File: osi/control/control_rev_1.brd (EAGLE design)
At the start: 25.4 x 25.4 mm, 8 parts, among them IC1 TINY24/44/84-PU

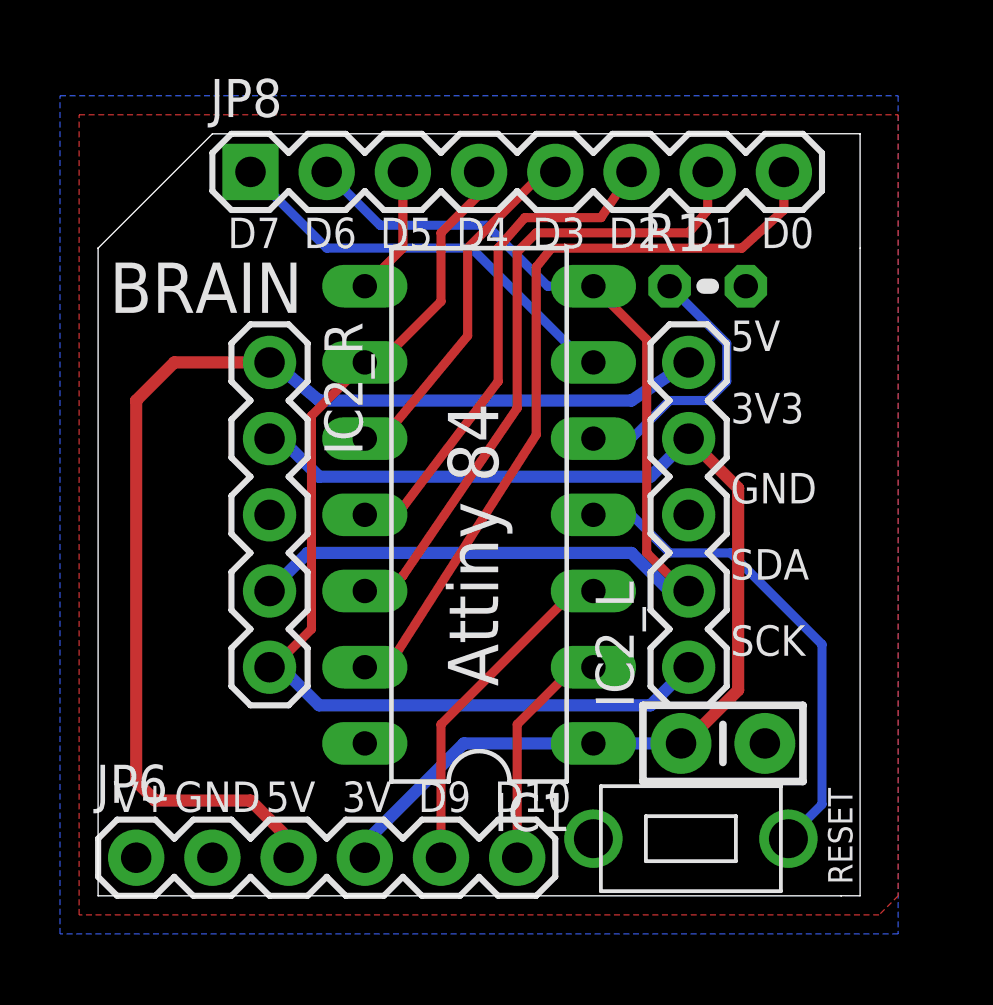
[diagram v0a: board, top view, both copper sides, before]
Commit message: control brain
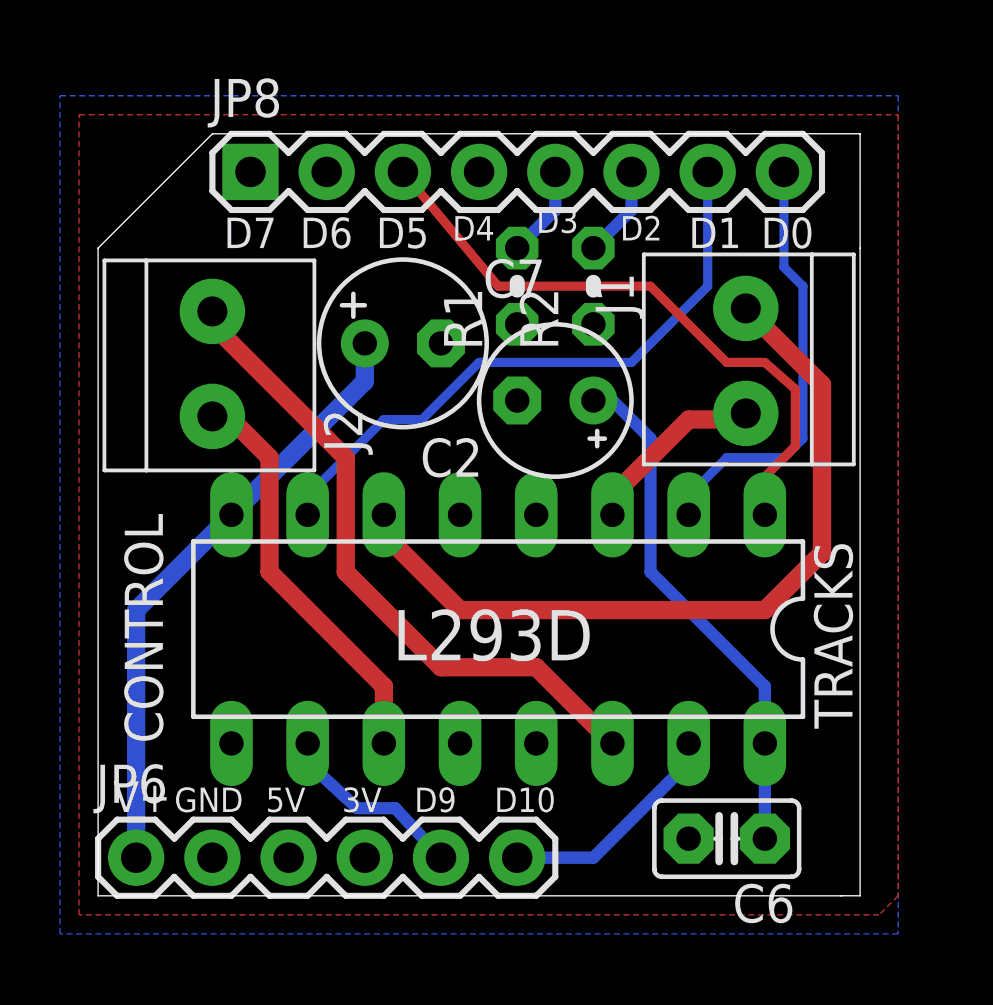
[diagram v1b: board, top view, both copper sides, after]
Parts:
- removed C1: (no value), SparkFun:CAP-PTH-SMALL-KIT
- removed IC1: TINY24/44/84-PU, avr-7:DIL14
- removed IC2_L, IC2_R: (no value), SparkFun_mod:1X05
- removed U$1: PTS635_SWITCH, _my-parts:PTS635_SWITCH
- added C2: 100uF/6V, rcl-ez:E2,5-5
- added C6: 0.1uF, rcl-ez:C025-025X050
- added C7: 100uF/16V, rcl-ez:E2,5-6
- added J1, J2: 1X2-3.5MM, adafruit_mod:1X2-3.5MM
- added R2: (no value), adafruit_mod:0204V
- added TRACKS: L293D, texas:DIL16
- moved R1 6.35 mm to (14.0, 20.3), turned to 90 degrees
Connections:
- removed net D8: IC1.5, R1.1
- removed net RESET: IC1.4, U$1.P$2
- new net N$1: J1.2, TRACKS.3
- new net N$2: J2.2, TRACKS.14
- new net N$3: J1.1, TRACKS.6
- new net N$4: J2.1, TRACKS.11
- new net N$5: TRACKS.9
- new net N$6: R1.1
- new net N$7: R2.1
- new net VCC: C2.+, C6.1, TRACKS.16
- net +3V3: no longer C1.2, IC1.1, IC2_L.4, IC2_R.2
- net +5V: no longer IC2_L.5, IC2_R.1
- net AREF_D0: now also TRACKS.2; no longer IC1.13
- net D1: now also TRACKS.7; no longer IC1.12
- net D10: now also TRACKS.15; no longer IC1.2
- net D2: now also R2.2; no longer IC1.11
- net D3: now also R1.2; no longer IC1.10
- net D5: now also TRACKS.1; no longer IC1.8
- net D7: no longer IC1.6
- net D9: now also TRACKS.10; no longer IC1.3
- net GND: now also C2.-, C6.2, C7.-, TRACKS.12, TRACKS.13, TRACKS.4, TRACKS.5; no longer C1.1, IC1.14, IC2_L.3, IC2_R.3, R1.2, U$1.P$1
- net SCL_D4: no longer IC1.9, IC2_L.1, IC2_R.5
- net SDA_D6: no longer IC1.7, IC2_L.2, IC2_R.4
- net V+: now also C7.+, TRACKS.8
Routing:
- net +3V3: track 39.4 -> 0.00 mm
- net +5V: track 39.0 -> 0.00 mm
- net SDA_D6: track 37.0 -> 0.00 mm
- net SCL_D4: track 34.8 -> 0.00 mm
- net N$3: track 0.00 -> 26.3 mm
- net N$2: track 0.00 -> 21.8 mm
- net V+: track 0.00 -> 20.3 mm
- net VCC: track 0.00 -> 17.3 mm
- net D5: track 4.34 -> 20.9 mm
- net RESET: track 16.3 -> 0.00 mm
- net D7: track 14.1 -> 0.00 mm
- net D2: track 16.8 -> 3.07 mm
- net N$4: track 0.00 -> 13.6 mm
- net AREF_D0: track 25.9 -> 14.4 mm
- net D8: track 9.20 -> 0.00 mm
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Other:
- board text added: "CONTROL"
- board text added: "Control Rev 1 Feb 12"
- board text added: "L293D"
- board text removed: "3V3"
- board text removed: "Attiny 84"
- board text removed: "BRAIN"
- board text removed: "Brain Rev 1 Feb 12"
- board text removed: "RESET"
- board text removed: "SCK"
- board text removed: "SDA"

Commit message: update
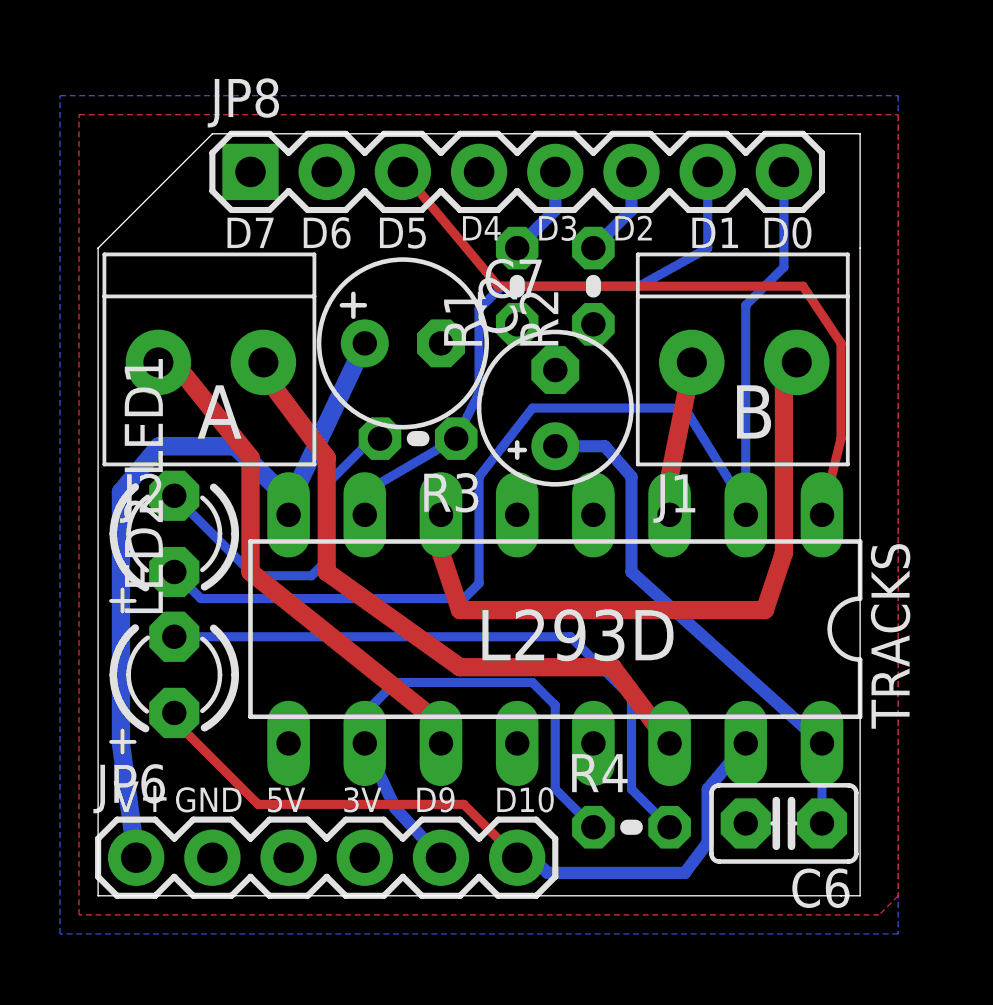
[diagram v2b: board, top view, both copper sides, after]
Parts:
- added LED1, LED2: (no value), adafruit:LED3MM
- added R3, R4: (no value), adafruit_mod:0204V
- moved C6 1.97 mm to (22.9, 2.41)
- moved TRACKS 1.90 mm to (15.2, 8.89)
- moved C2 0.25 mm to (15.2, 16.3), turned to 90 degrees
- turned J1 to 180 degrees
- turned J2 to 180 degrees
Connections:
- net AREF_D0: now also LED1.A
- net D1: now also R3.1
- net D10: now also LED2.A
- net D9: now also R4.1
- net GND: now also R1.1, R2.1
- net N$1: now also J1.1; no longer J1.2
- net N$3: now also J1.2; no longer J1.1
- net N$6: now also LED1.K, R3.2; no longer R1.1
- net N$7: now also LED2.K, R4.2; no longer R2.1
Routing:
- net AREF_D0: track 14.4 -> 38.1 mm
- net N$7: track 0.00 -> 20.9 mm
- net D10: track 7.67 -> 24.4 mm
- net N$6: track 0.00 -> 11.3 mm
- net D9: track 6.40 -> 17.3 mm
- net V+: track 20.3 -> 27.1 mm
- net N$3: track 26.3 -> 21.9 mm
- net N$4: track 13.6 -> 17.2 mm
- net D5: track 20.9 -> 23.2 mm
- net D1: track 20.7 -> 19.6 mm
- net N$1: track 6.22 -> 5.19 mm
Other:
- board text added: "A"
- board text added: "B"
- board text added: "Rev 1 Feb 12"
- board text removed: "Control Rev 1 Feb 12"
